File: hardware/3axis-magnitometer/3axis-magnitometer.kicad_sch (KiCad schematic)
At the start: 12 parts, among them J1 Conn_01x08_Pin

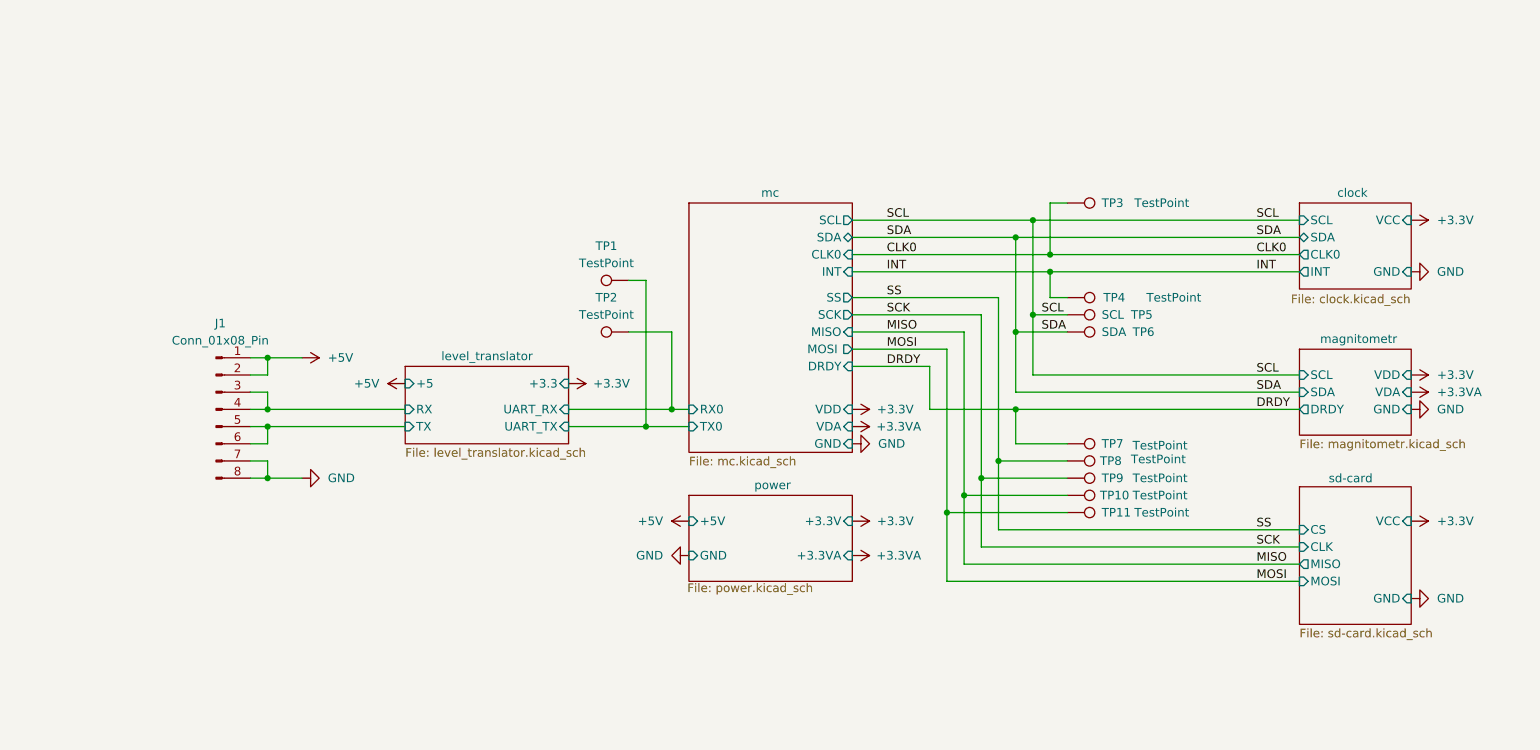
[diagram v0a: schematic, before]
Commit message: Add files via upload
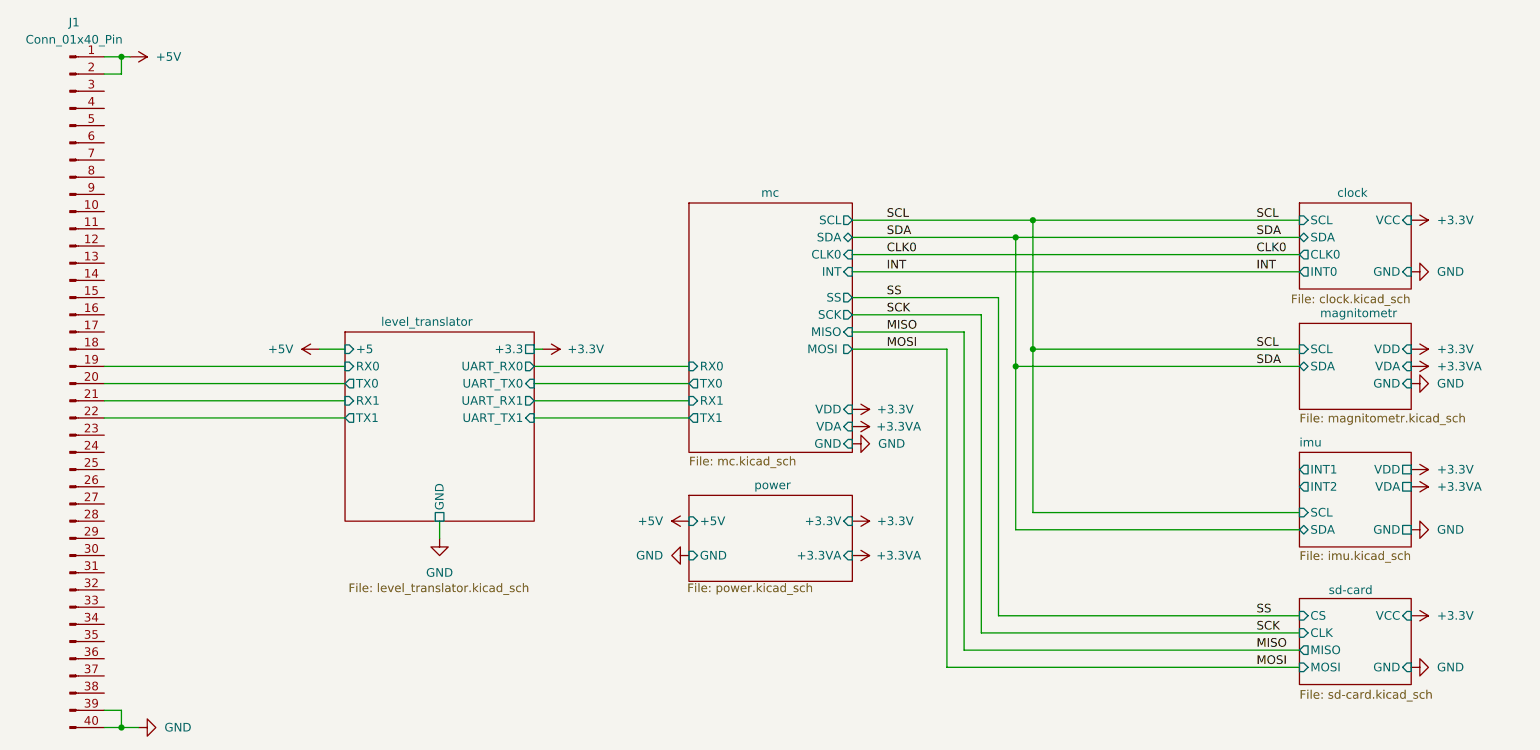
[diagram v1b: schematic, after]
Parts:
- removed J1: Conn_01x08_Pin, Connector_PinHeader_2.54mm:PinHeader_2x04_P2.54mm_Vertical, symbol Connector:Conn_01x08_Pin
- removed TP1, TP10, TP11, TP2, TP3, TP4, TP7, TP8, TP9: TestPoint, TestPoint:TestPoint_Pad_D1.0mm, symbol Connector:TestPoint
- removed TP5: SCL, TestPoint:TestPoint_Pad_D1.0mm, symbol Connector:TestPoint
- removed TP6: SDA, TestPoint:TestPoint_Pad_D1.0mm, symbol Connector:TestPoint
- added J1: Conn_01x40_Pin, symbol Connector:Conn_01x40_Pin
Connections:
- net +5V: now also J1.1 (Pin_1), J1.2 (Pin_2)
- net GND: now also J1.39 (Pin_39), J1.40 (Pin_40)
- new net level_translator/RX0: J1.19 (Pin_19)
- new net level_translator/RX1: J1.21 (Pin_21)
- new net level_translator/TX0: J1.20 (Pin_20)
- new net level_translator/TX1: J1.22 (Pin_22)
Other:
- added sheet imu (imu.kicad_sch)
- sheet clock ports: added INT0; removed INT
- sheet level_translator ports: added GND, RX0, RX1, TX0, TX1, UART_RX0, UART_RX1, UART_TX0, UART_TX1; removed RX, TX, UART_RX, UART_TX
- sheet magnitometr ports: added none; removed DRDY
- sheet mc ports: added RX1, TX1; removed DRDY

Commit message: начата новая трассировка
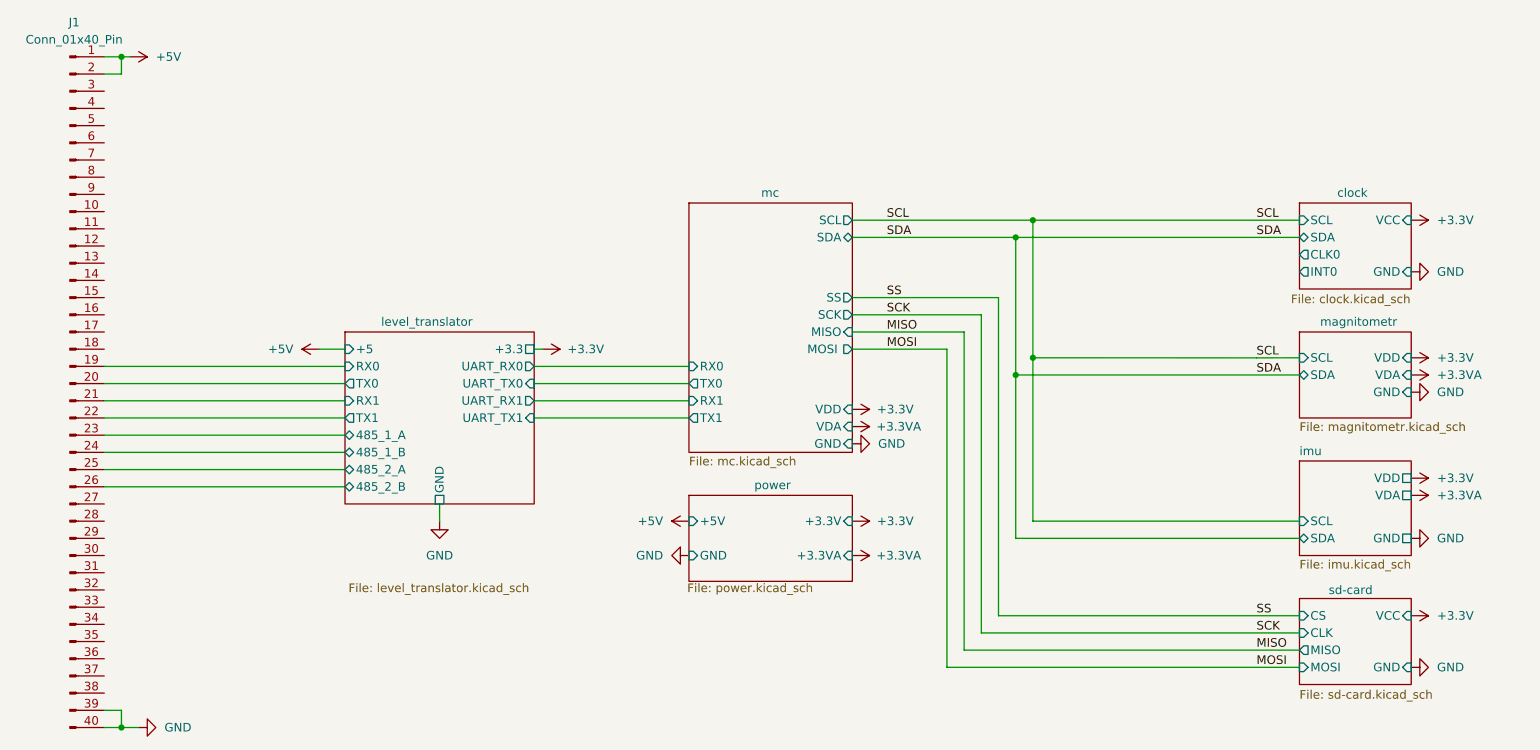
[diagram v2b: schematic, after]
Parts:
- J1: footprint (none) -> Connector_PinHeader_2.54mm:PinHeader_2x20_P2.54mm_Horizontal
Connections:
- net level_translator/485_1_A: now reaches J1.23 (Pin_23)
- net level_translator/485_1_B: now reaches J1.24 (Pin_24)
- net level_translator/485_2_A: now reaches J1.25 (Pin_25)
- net level_translator/485_2_B: now reaches J1.26 (Pin_26)
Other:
- sheet imu ports: added none; removed INT1, INT2
- sheet level_translator ports: added 485_1_A, 485_1_B, 485_2_A, 485_2_B; removed none
- sheet mc ports: added none; removed CLK0, INT
